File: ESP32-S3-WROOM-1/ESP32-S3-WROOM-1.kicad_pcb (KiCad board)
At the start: 2 copper layers, 25.4 x 57 mm, 23 parts, among them J1 ESP32-S3-DEVKITC-1-J1, J2 ESP32-S3-DEVKITC-1-J2, J3 UART, P1 USB2.0_C_12pin, SW1 BOOT, SW2 RESET, U1 ESP32-S3-WROOM-1, U2 AMS1117-3.3

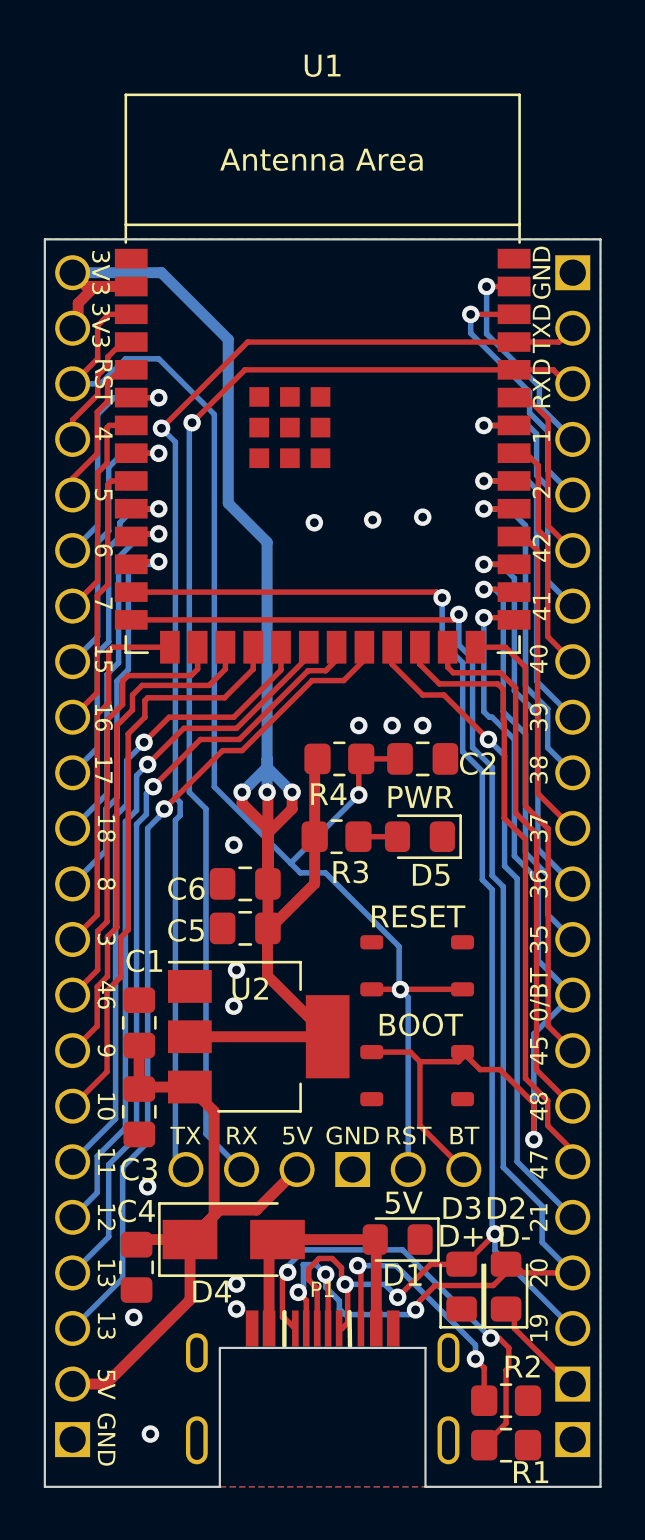
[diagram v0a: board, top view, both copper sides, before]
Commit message: order
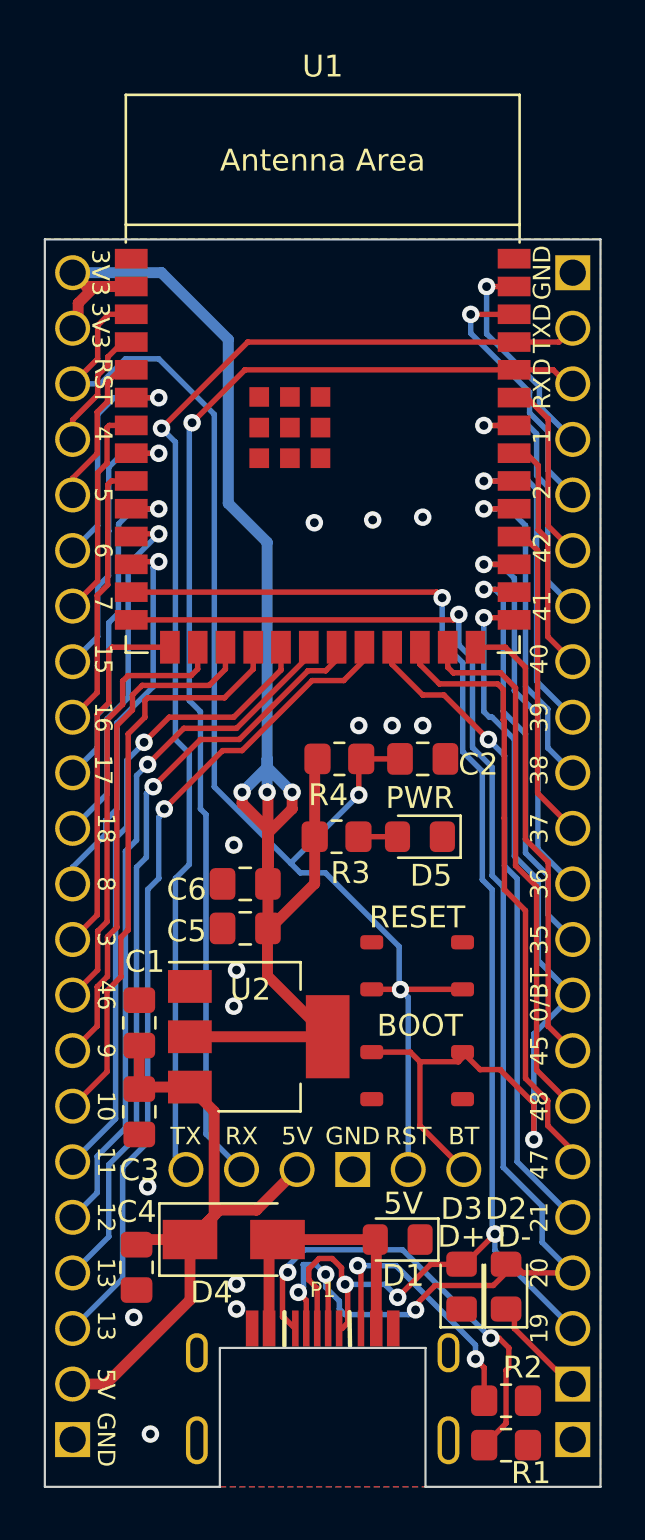
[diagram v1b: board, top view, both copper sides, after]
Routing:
- net GPIO8: track 18.3 -> 17.7 mm
